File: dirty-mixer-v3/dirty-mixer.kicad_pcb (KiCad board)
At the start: 2 copper layers, 15 x 98 mm, 8 parts, among them J1 AudioJack2_SwitchT, J2 AudioJack2_SwitchT, J3 AudioJack2_SwitchT, J4 AudioJack2_SwitchT, J5 AudioJack2_SwitchT, SW1 SW_SPDT, SW2 SW_SPDT

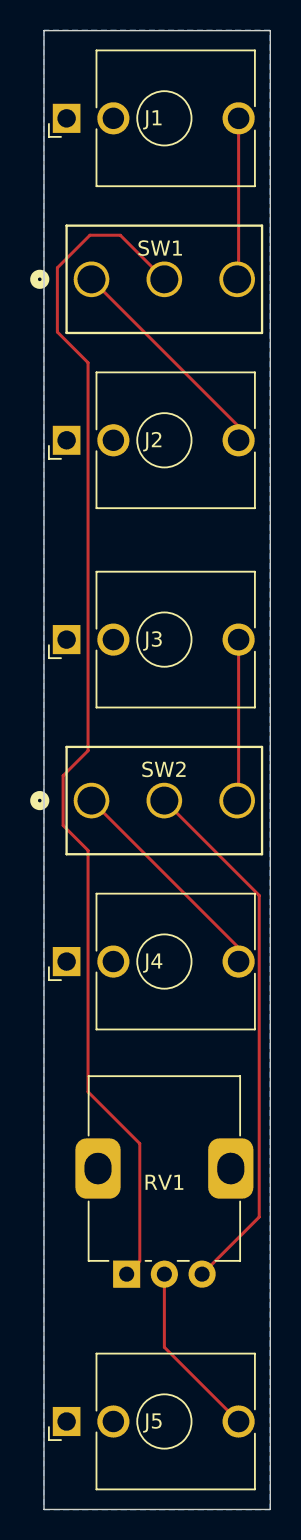
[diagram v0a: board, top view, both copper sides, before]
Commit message: some pcb changes
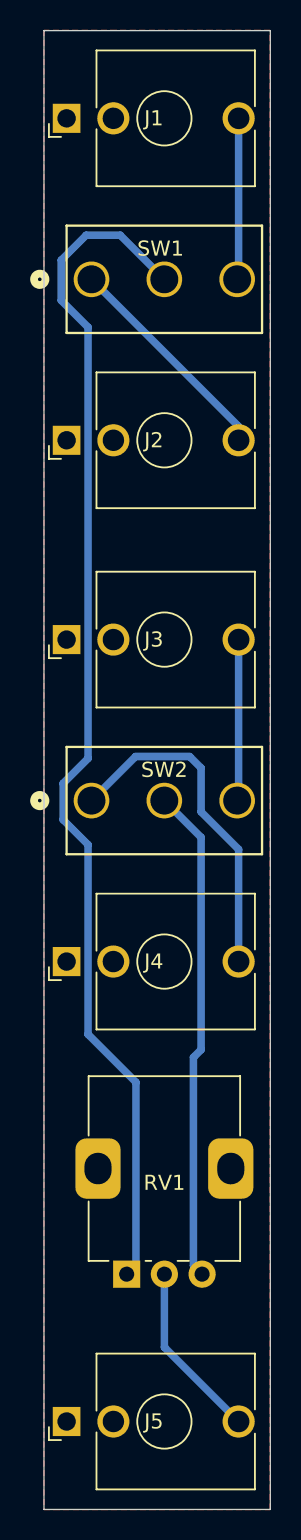
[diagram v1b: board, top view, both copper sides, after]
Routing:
- net Net-(SW2-A): track 14.7 -> 22.6 mm
- net Net-(SW2-B): track 35.6 -> 32.8 mm
- added copper zone on F.Cu, net GND
- removed copper zone on B.Cu, net GND
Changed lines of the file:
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@@
 		(start 104.75 82.804)
 		(end 114.5 92.554)
-		(width 0.2)
-		(layer "F.Cu")
+		(width 0.5)
+		(layer "B.Cu")
 		(net 2)
 	)
@@
 		(start 114.5 92.554)
 		(end 114.5 93.472)
-		(width 0.2)
-		(layer "F.Cu")
+		(width 0.5)
+		(layer "B.Cu")
 		(net 2)
 	)
@@
 		(start 114.5 72.136)
 		(end 114.5 82.706)
-		(width 0.2)
-		(layer "F.Cu")
+		(width 0.5)
+		(layer "B.Cu")
 		(net 4)
 	)
@@
 		(start 114.5 82.706)
 		(end 114.402 82.804)
-		(width 0.2)
-		(layer "F.Cu")
+		(width 0.5)
+		(layer "B.Cu")
 		(net 4)
 	)
 	(segment
-		(start 114.5 127.098)
+		(start 112.014 118.093069)
+		(end 114.5 120.579069)
+		(width 0.5)
+		(layer "B.Cu")
+		(net 6)
+	)
+	(segment
+		(start 107.671 114.427)
+		(end 111.252 114.427)
+		(width 0.5)
+		(layer "B.Cu")
+		(net 6)
+	)
+	(segment
+		(start 111.252 114.427)
+		(end 112.014 115.189)
+		(width 0.5)
+		(layer "B.Cu")
+		(net 6)
+	)
+	(segment
+		(start 112.014 115.189)
+		(end 112.014 118.093069)
+		(width 0.5)
+		(layer "B.Cu")
+		(net 6)
+	)
+	(segment
+		(start 104.75 117.348)
+		(end 107.671 114.427)
+		(width 0.5)
+		(layer "B.Cu")
+		(net 6)
+	)
+	(segment
+		(start 114.5 120.579069)
 		(end 114.5 128.016)
-		(width 0.2)
-		(layer "F.Cu")
-		(net 6)
-	)
-	(segment
-		(start 104.75 117.348)
-		(end 114.5 127.098)
-		(width 0.2)
-		(layer "F.Cu")
+		(width 0.5)
+		(layer "B.Cu")
 		(net 6)
 	)
@@
 		(start 114.5 117.25)
 		(end 114.402 117.348)
-		(width 0.2)
-		(layer "F.Cu")
+		(width 0.5)
+		(layer "B.Cu")
 		(net 8)
 	)
@@
 		(start 114.5 106.68)
 		(end 114.5 117.25)
-		(width 0.2)
-		(layer "F.Cu")
+		(width 0.5)
+		(layer "B.Cu")
 		(net 8)
 	)
@@
 		(start 109.58 153.576)
 		(end 114.5 158.496)
-		(width 0.2)
-		(layer "F.Cu")
+		(width 0.5)
+		(layer "B.Cu")
 		(net 10)
 	)
@@
 		(start 109.58 148.732)
 		(end 109.58 153.576)
-		(width 0.2)
-		(layer "F.Cu")
+		(width 0.5)
+		(layer "B.Cu")
 		(net 10)
 	)
 	(segment
-		(start 104.521 114.046)
-		(end 102.87 115.697)
-		(width 0.2)
-		(layer "F.Cu")
-		(net 12)
-	)
-	(segment
-		(start 104.521 120.65)
-		(end 104.521 136.652)
-		(width 0.2)
-		(layer "F.Cu")
-		(net 12)
-	)
-	(segment
-		(start 104.521 88.3285)
-		(end 104.521 114.046)
-		(width 0.2)
-		(layer "F.Cu")
+		(start 102.87 116.205)
+		(end 102.87 118.618)
+		(width 0.5)
+		(layer "B.Cu")
+		(net 12)
+	)
+	(segment
+		(start 104.521 132.842)
+		(end 107.696 136.017)
+		(width 0.5)
+		(layer "B.Cu")
+		(net 12)
+	)
+	(segment
+		(start 106.655 79.883)
+		(end 104.394 79.883)
+		(width 0.5)
+		(layer "B.Cu")
 		(net 12)
 	)
@@
 		(start 109.576 82.804)
 		(end 106.655 79.883)
-		(width 0.2)
-		(layer "F.Cu")
-		(net 12)
-	)
-	(segment
-		(start 106.655 79.883)
-		(end 104.648 79.883)
-		(width 0.2)
-		(layer "F.Cu")
-		(net 12)
-	)
-	(segment
-		(start 104.521 136.652)
-		(end 107.95 140.081)
-		(width 0.2)
-		(layer "F.Cu")
-		(net 12)
-	)
-	(segment
-		(start 107.95 147.862)
+		(width 0.5)
+		(layer "B.Cu")
+		(net 12)
+	)
+	(segment
+		(start 102.87 118.618)
+		(end 104.521 120.269)
+		(width 0.5)
+		(layer "B.Cu")
+		(net 12)
+	)
+	(segment
+		(start 104.521 120.269)
+		(end 104.521 132.842)
+		(width 0.5)
+		(layer "B.Cu")
+		(net 12)
+	)
+	(segment
+		(start 104.521 85.979)
+		(end 104.521 114.554)
+		(width 0.5)
+		(layer "B.Cu")
+		(net 12)
+	)
+	(segment
+		(start 107.696 148.116)
 		(end 107.08 148.732)
-		(width 0.2)
-		(layer "F.Cu")
-		(net 12)
-	)
-	(segment
-		(start 107.95 140.081)
-		(end 107.95 147.862)
-		(width 0.2)
-		(layer "F.Cu")
-		(net 12)
-	)
-	(segment
-		(start 102.87 115.697)
-		(end 102.87 118.999)
-		(width 0.2)
-		(layer "F.Cu")
-		(net 12)
-	)
-	(segment
-		(start 102.489 82.042)
-		(end 102.489 86.2965)
-		(width 0.2)
-		(layer "F.Cu")
-		(net 12)
-	)
-	(segment
-		(start 102.489 86.2965)
-		(end 104.521 88.3285)
-		(width 0.2)
-		(layer "F.Cu")
-		(net 12)
-	)
-	(segment
-		(start 104.648 79.883)
-		(end 102.489 82.042)
-		(width 0.2)
-		(layer "F.Cu")
-		(net 12)
-	)
-	(segment
-		(start 102.87 118.999)
-		(end 104.521 120.65)
-		(width 0.2)
-		(layer "F.Cu")
-		(net 12)
-	)
-	(segment
-		(start 115.865 144.947)
+		(width 0.5)
+		(layer "B.Cu")
+		(net 12)
+	)
+	(segment
+		(start 102.743 84.201)
+		(end 104.521 85.979)
+		(width 0.5)
+		(layer "B.Cu")
+		(net 12)
+	)
+	(segment
+		(start 104.521 114.554)
+		(end 102.87 116.205)
+		(width 0.5)
+		(layer "B.Cu")
+		(net 12)
+	)
+	(segment
+		(start 102.743 81.534)
+		(end 102.743 84.201)
+		(width 0.5)
+		(layer "B.Cu")
+		(net 12)
+	)
+	(segment
+		(start 107.696 136.017)
+		(end 107.696 148.116)
+		(width 0.5)
+		(layer "B.Cu")
+		(net 12)
+	)
+	(segment
+		(start 104.394 79.883)
+		(end 102.743 81.534)
+		(width 0.5)
+		(layer "B.Cu")
+		(net 12)
+	)
+	(segment
+		(start 109.576 117.348)
+		(end 112.014 119.786)
+		(width 0.5)
+		(layer "B.Cu")
+		(net 13)
+	)
+	(segment
+		(start 112.014 133.858)
+		(end 111.506 134.366)
+		(width 0.5)
+		(layer "B.Cu")
+		(net 13)
+	)
+	(segment
+		(start 111.506 148.158)
 		(end 112.08 148.732)
-		(width 0.2)
-		(layer "F.Cu")
-		(net 13)
-	)
-	(segment
-		(start 115.865 123.637)
-		(end 115.865 144.947)
-		(width 0.2)
-		(layer "F.Cu")
-		(net 13)
-	)
-	(segment
-		(start 109.576 117.348)
-		(end 115.865 123.637)
-		(width 0.2)
-		(layer "F.Cu")
+		(width 0.5)
+		(layer "B.Cu")
+		(net 13)
+	)
+	(segment
+		(start 112.014 119.786)
+		(end 112.014 133.858)
+		(width 0.5)
+		(layer "B.Cu")
+		(net 13)
+	)
+	(segment
+		(start 111.506 134.366)
+		(end 111.506 148.158)
+		(width 0.5)
+		(layer "B.Cu")
 		(net 13)
 	)
@@
 		(net 3)
 		(net_name "GND")
-		(layer "B.Cu")
+		(layer "F.Cu")
 		(hatch edge 0.5)
 		(connect_pads yes
